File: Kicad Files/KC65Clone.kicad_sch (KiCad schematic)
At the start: 22 parts, among them J1 Conn_01x04, SW76 SKQGABE010, SW77 SKQGABE010, U1 STM32F072C8Tx, U2 XC6206P332MR

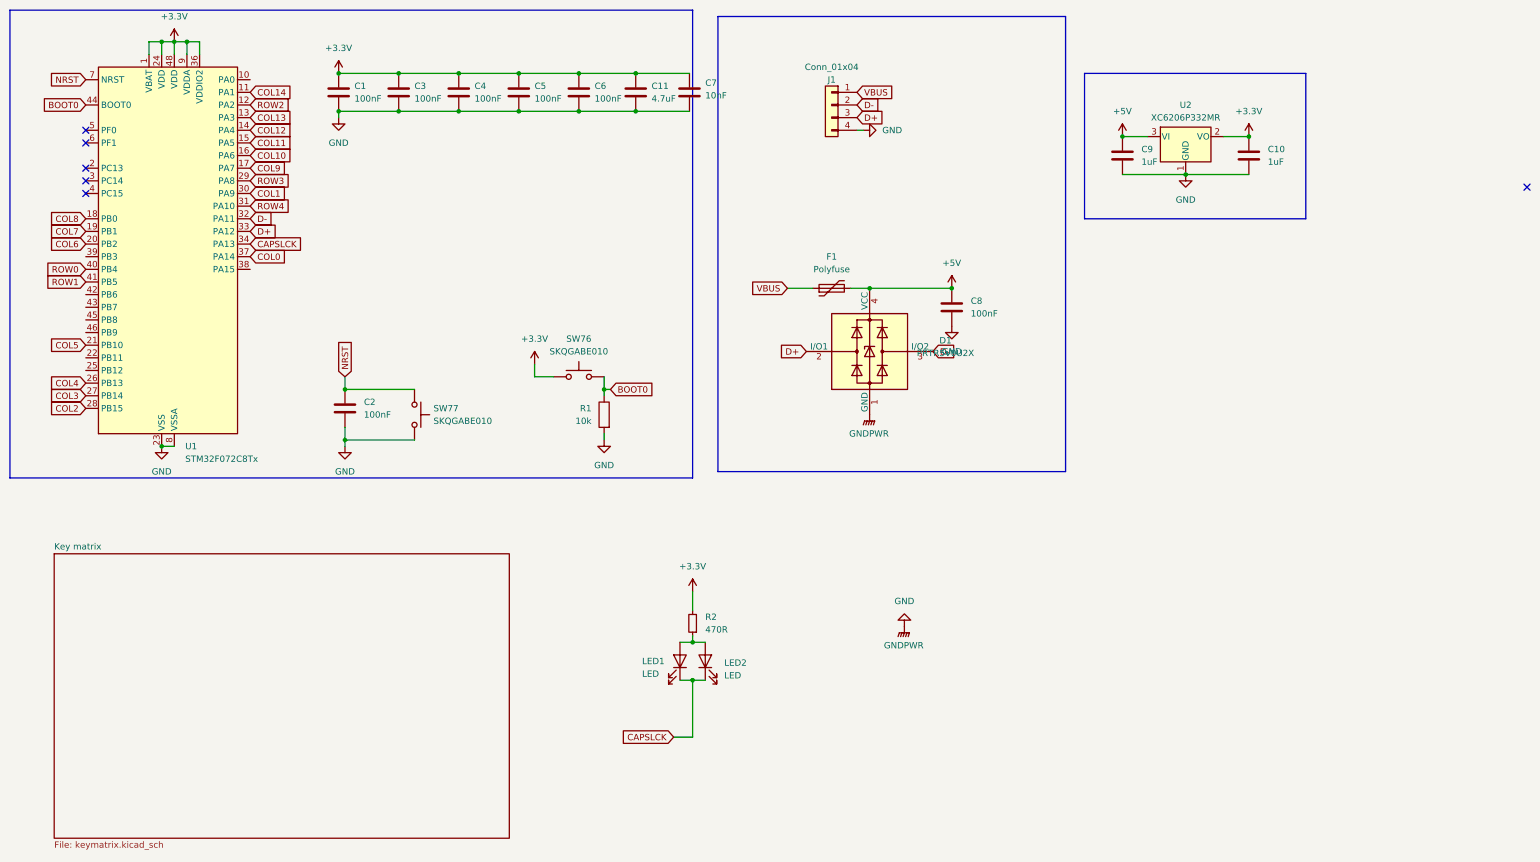
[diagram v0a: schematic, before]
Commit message: added holes
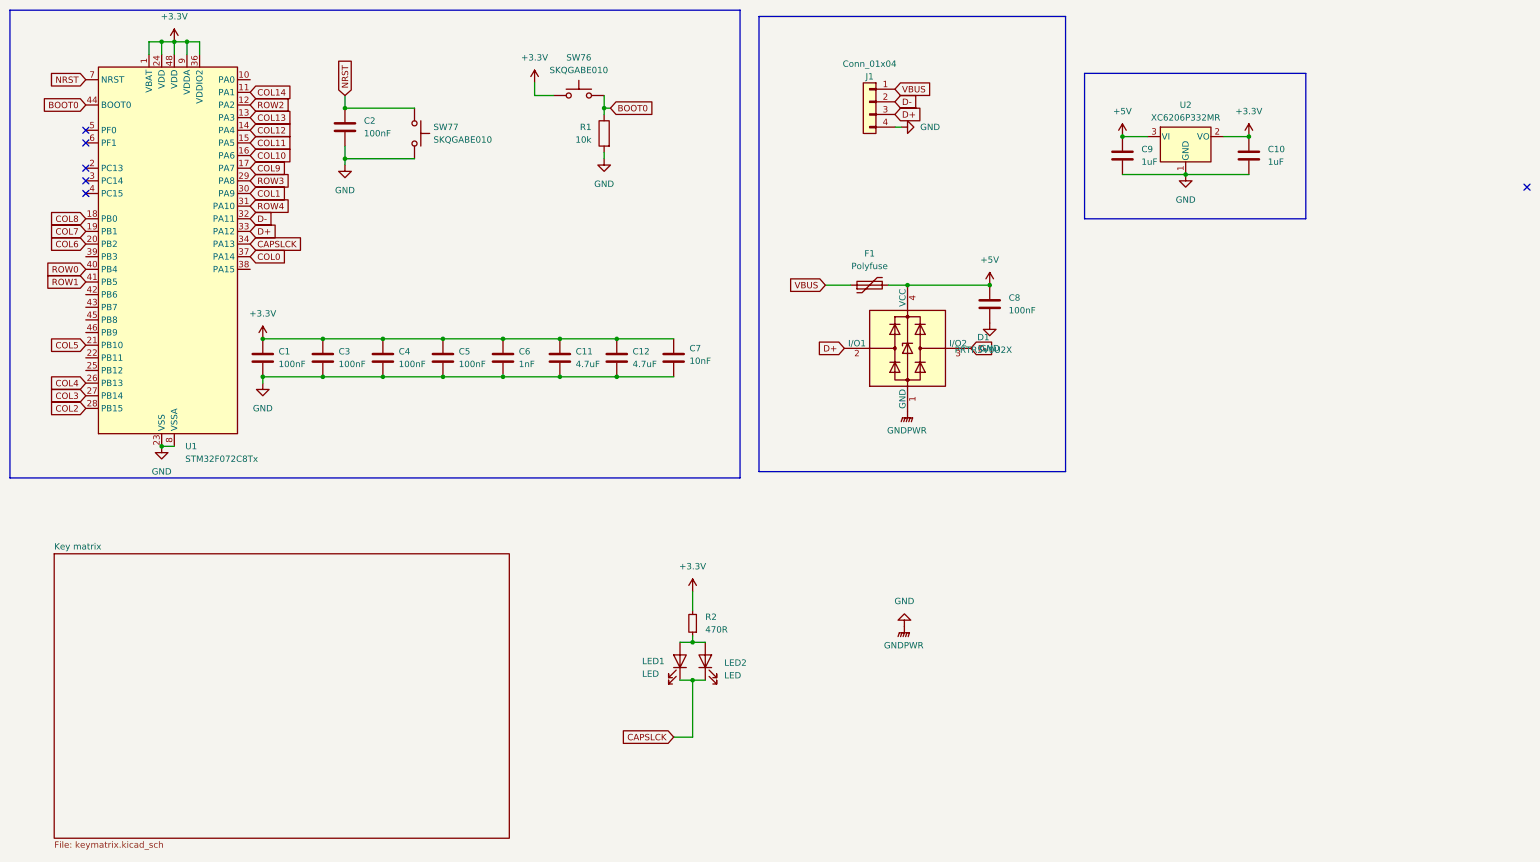
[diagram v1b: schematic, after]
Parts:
- added C12: 4.7uF, Capacitor_SMD:C_0402_1005Metric, symbol Device:C
- C6: value 100nF -> 1nF
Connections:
- net +3.3V: now also C12.1
- net GND: now also C12.2
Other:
- moved on the sheet: C1, C11, C2, C3, C4, C5, C6, C7, C8, D1, F1, J1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
